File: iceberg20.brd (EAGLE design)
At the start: 210 x 172.5 mm, 210 parts, among them K1:C1 2,2 mF, 16 V, ±20 %, K1:D1 DIODE, K1:R1 300R, K1:R2 100k, K1:T1 IRF1405, M0:+ TPB1,27, M0:- TPB1,27, M0:C1 10nF, M0:C2 220nF, M0:C3 100nF, M0:C4 100uF, 16V, ±20 %, M0:C5 1nF, M0:C6 100nF, M0:D1 DIODE, M0:D2 DIODE, M0:EN TPB1,27, M0:I TPB1,27, M0:IC1 L6205N, M0:IC2 ACS712ACS712-SOIC-8, M0:IN1 TPB1,27, M0:IN2 TPB1,27, M0:R1 100R, M0:R2 100k, M0:R3 10k, M0:VS TPB1,27, M1:+ TPB1,27, M1:- TPB1,27, M1:C1 10nF, M1:C2 220nF, M1:C3 100nF, M1:C4 100uF, 16V, ±20 %, M1:C5 1nF, M1:C6 100nF, M1:D1 DIODE, M1:D2 DIODE, M1:EN TPB1,27, M1:I TPB1,27, M1:IC1 L6205N, M1:IC2 ACS712ACS712-SOIC-8, M1:IN1 TPB1,27, M1:IN2 TPB1,27, M1:R1 100R, M1:R2 100k, M1:R3 10k, M1:VS TPB1,27, M2:+ TPB1,27, M2:- TPB1,27, M2:C1 10nF, M2:C2 220nF, M2:C3 100nF, M2:C4 100uF, 16V, ±20 %, M2:C5 1nF, M2:C6 100nF, M2:D1 DIODE, M2:D2 DIODE, M2:EN TPB1,27, M2:I TPB1,27, M2:IC1 L6205N, M2:IC2 ACS712ACS712-SOIC-8, M2:IN1 TPB1,27, M2:IN2 TPB1,27, M2:R1 100R, M2:R2 100k, M2:R3 10k, M2:VS TPB1,27, M3:+ TPB1,27, M3:- TPB1,27, M3:C1 10nF, M3:C2 220nF, M3:C3 100nF, M3:C4 100uF, 16V, ±20 %, M3:C5 1nF, M3:C6 100nF, M3:D1 DIODE, M3:D2 DIODE, M3:EN TPB1,27, M3:I TPB1,27, M3:IC1 L6205N, M3:IC2 ACS712ACS712-SOIC-8, M3:IN1 TPB1,27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

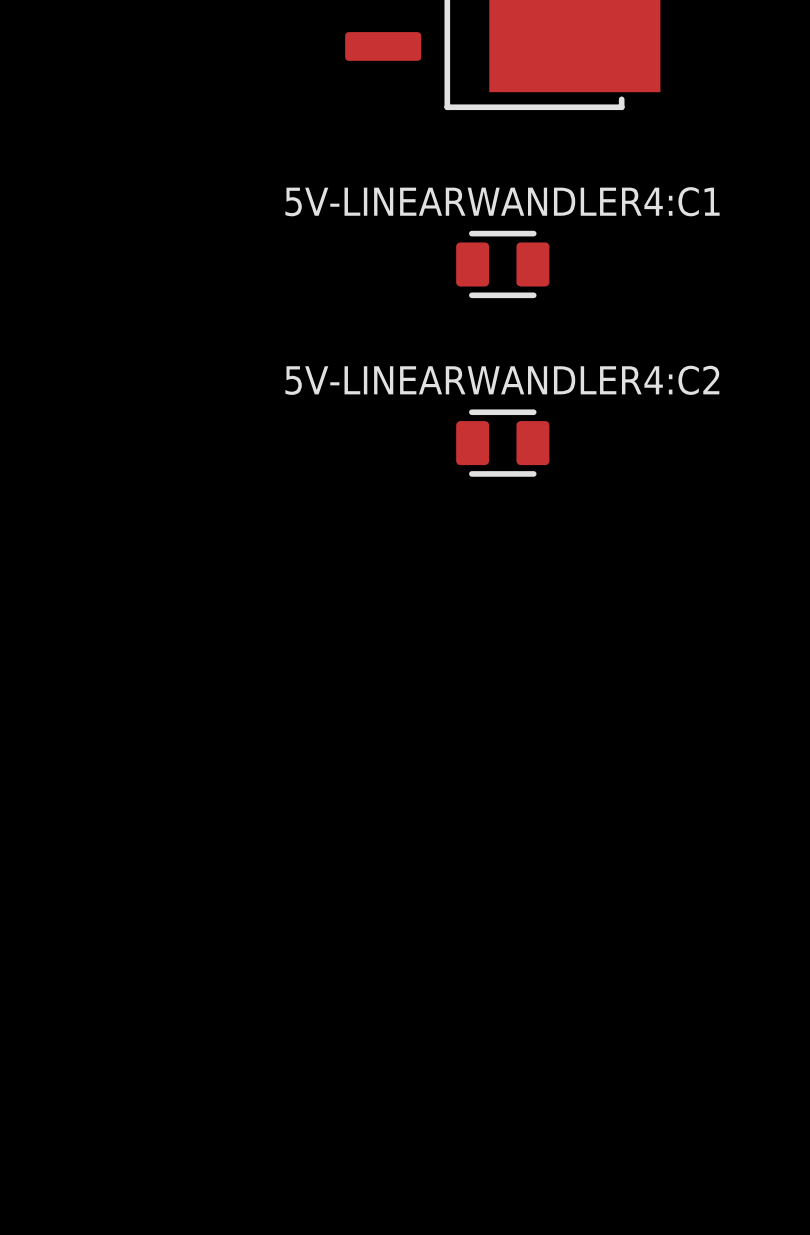
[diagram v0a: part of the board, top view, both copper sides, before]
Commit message: + sch (Bus Buffer)
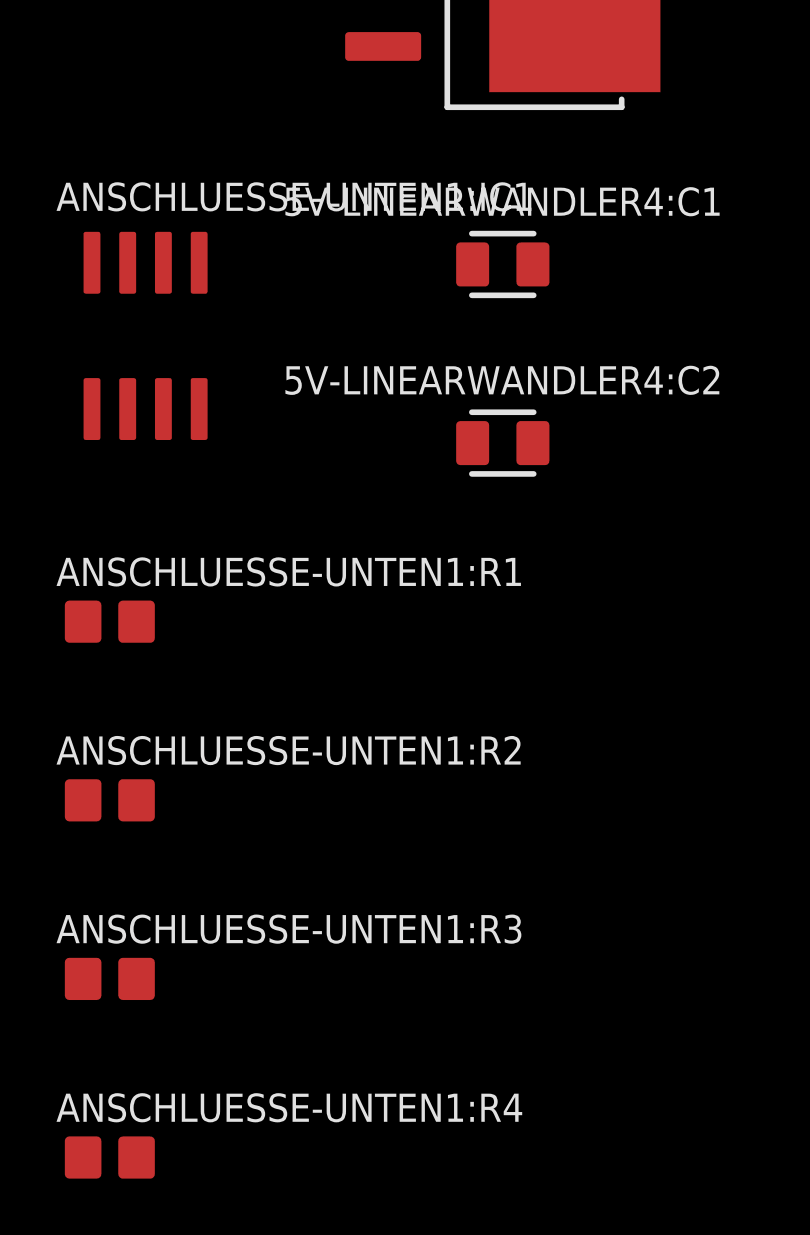
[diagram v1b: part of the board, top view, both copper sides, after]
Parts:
- added ANSCHLUESSE-UNTEN1:IC1: P82B96, iceberg20:SO8
- added ANSCHLUESSE-UNTEN1:R1, ANSCHLUESSE-UNTEN1:R2, ANSCHLUESSE-UNTEN1:R3, ANSCHLUESSE-UNTEN1:R4: 10k, iceberg20:R0805
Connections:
- new net ANSCHLUESSE-UNTEN1:RX(SDA): ANSCHLUESSE-UNTEN1:IC1.2, ANSCHLUESSE-UNTEN1:R3.1, ANSCHLUESSE-UNTEN1:X2.23
- new net ANSCHLUESSE-UNTEN1:RY(SCL): ANSCHLUESSE-UNTEN1:IC1.6, ANSCHLUESSE-UNTEN1:R4.1, ANSCHLUESSE-UNTEN1:X2.26
- new net ANSCHLUESSE-UNTEN1:TX(SDA): ANSCHLUESSE-UNTEN1:IC1.3, ANSCHLUESSE-UNTEN1:R2.1, ANSCHLUESSE-UNTEN1:X2.22
- new net ANSCHLUESSE-UNTEN1:TY(SCL): ANSCHLUESSE-UNTEN1:IC1.5, ANSCHLUESSE-UNTEN1:R1.1, ANSCHLUESSE-UNTEN1:X2.25
- net ANSCHLUSS: now also ANSCHLUESSE-UNTEN1:IC1.8, ANSCHLUESSE-UNTEN1:R1.2, ANSCHLUESSE-UNTEN1:R2.2, ANSCHLUESSE-UNTEN1:R3.2, ANSCHLUESSE-UNTEN1:R4.2
- net GND: now also ANSCHLUESSE-UNTEN1:IC1.4; no longer ANSCHLUESSE-UNTEN1:X2.22, ANSCHLUESSE-UNTEN1:X2.25
- net SCL: now also ANSCHLUESSE-UNTEN1:IC1.7; no longer ANSCHLUESSE-UNTEN1:X2.26
- net SDA: now also ANSCHLUESSE-UNTEN1:IC1.1; no longer ANSCHLUESSE-UNTEN1:X2.23
